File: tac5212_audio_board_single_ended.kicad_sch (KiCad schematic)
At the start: 94 parts, among them J1002 TAC5212, U1 Single Buffer - 74LVC1G125GV,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, U2 3.3v LDO - TLV74133PDBVR

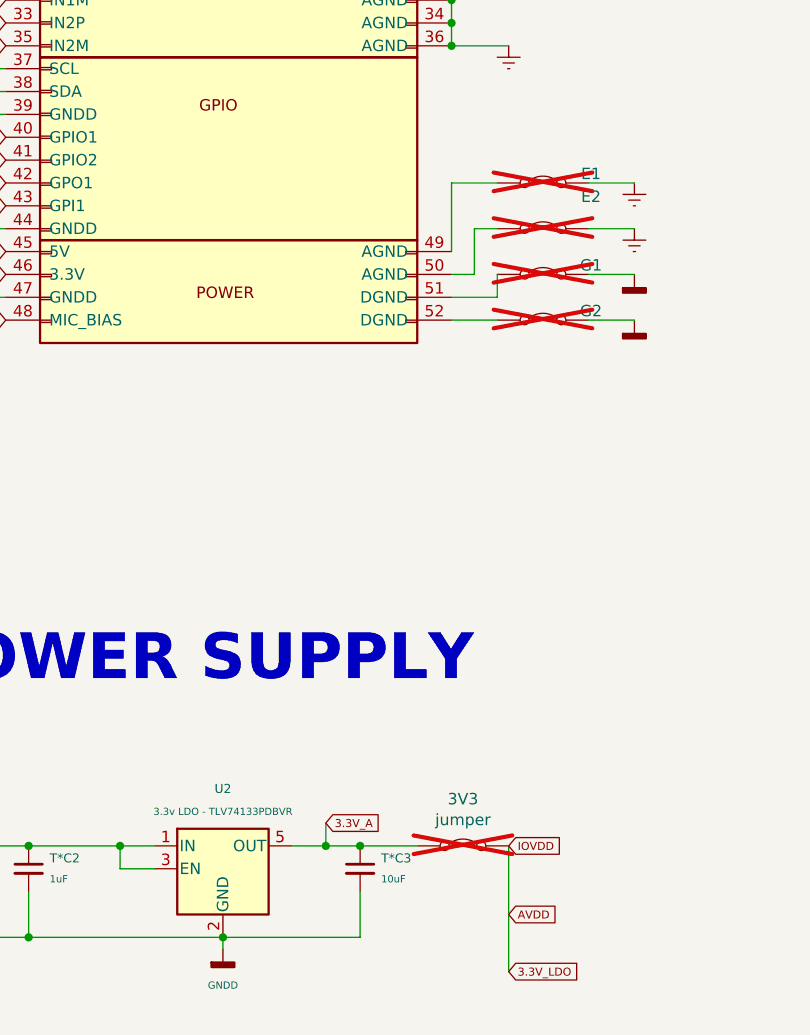
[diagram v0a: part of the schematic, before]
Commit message: UPDATE
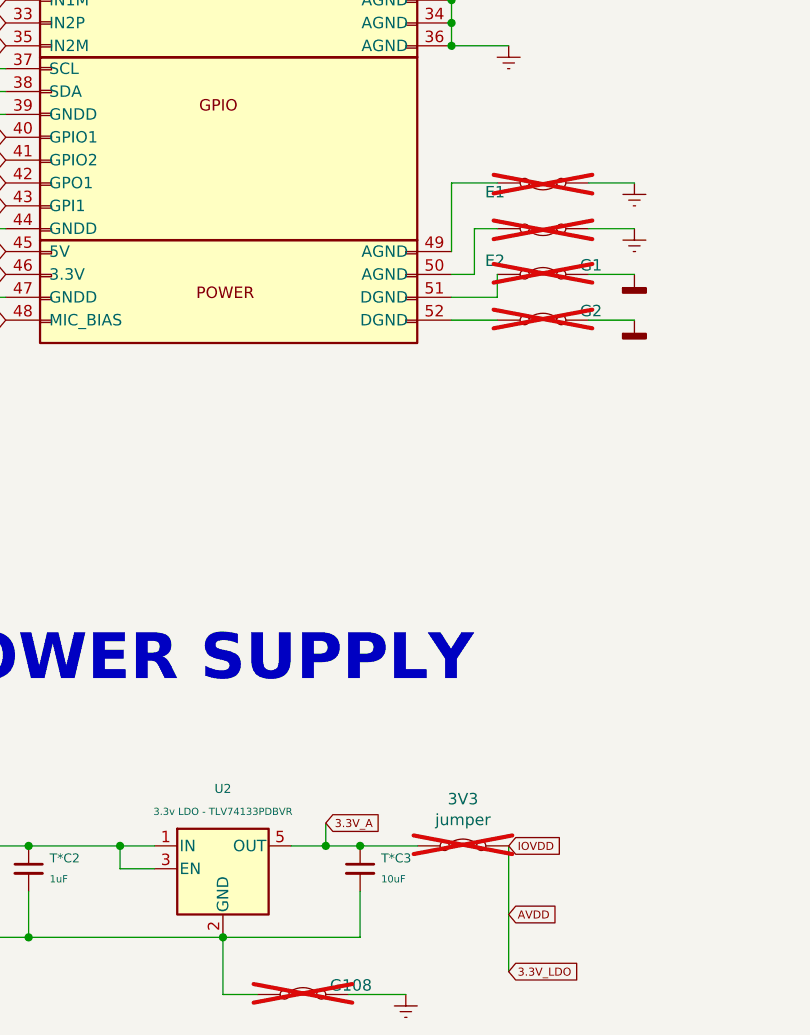
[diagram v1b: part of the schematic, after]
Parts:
- added G108: jumper, project_fp:jumper_slice, symbol proejct_lib:Jumper_2_Bridged
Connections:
- net Earth: now also E1.1 (A), E2.1 (A), G108.2 (B); no longer E1.2 (B), E2.2 (B)
- net GNDD: no longer T*C1.2, T*C2.2, T*C3.2, U2.2 (GND)
- net at board_outline1.49 (AGND): now also E1.2 (B); no longer E1.1 (A)
- net at board_outline1.50 (AGND): now also E2.2 (B); no longer E2.1 (A)
- new net: G108.1 (A), T*C1.2, T*C2.2, T*C3.2, U2.2 (GND)
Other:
- moved on the sheet: E1, E2
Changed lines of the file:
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@@
 	(wire
 		(pts
+			(xy 110.49 372.11) (xy 104.14 372.11)
+		)
+		(stroke
+			(width 0)
+			(type default)
+		)
+	)
+	(wire
+		(pts
 			(xy 218.44 168.91) (xy 222.25 168.91)
 		)
@@
 	(wire
 		(pts
-			(xy 90.17 367.03) (xy 90.17 365.76)
-		)
-		(stroke
-			(width 0)
-			(type default)
-		)
-	)
-	(wire
-		(pts
 			(xy 190.5 91.44) (xy 199.39 91.44)
 		)
@@
 	(wire
 		(pts
+			(xy 90.17 372.11) (xy 93.98 372.11)
+		)
+		(stroke
+			(width 0)
+			(type default)
+		)
+	)
+	(wire
+		(pts
 			(xy 49.53 294.64) (xy 66.04 294.64)
 		)
@@
 	(wire
 		(pts
+			(xy 90.17 372.11) (xy 90.17 365.76)
+		)
+		(stroke
+			(width 0)
+			(type default)
+		)
+	)
+	(wire
+		(pts
 			(xy 71.12 156.21) (xy 71.12 157.48)
 		)
@@
 	)
 	(symbol
+		(lib_id "proejct_lib:Earth")
+		(at 110.49 372.11 0)
+		(mirror y)
+		(unit 1)
+		(exclude_from_sim no)
+		(in_bom yes)
+		(on_board yes)
+		(dnp no)
+		(fields_autoplaced yes)
+		(property "Reference" "#PWR0108"
+			(at 110.49 378.46 0)
+			(effects
+				(font
+					(size 1 1)
+				)
+				(hide yes)
+			)
+		)
+		(property "Value" "Earth"
+			(at 110.49 375.92 0)
+			(effects
+				(font
+					(size 0.8 0.8)
+				)
+				(hide yes)
+			)
+		)
+		(property "Footprint" ""
+			(at 110.49 372.11 0)
+			(effects
+				(font
+					(size 0.8 0.8)
+				)
+				(hide yes)
+			)
+		)
+		(property "Datasheet" "~"
+			(at 110.49 372.11 0)
+			(effects
+				(font
+					(size 0.8 0.8)
+				)
+				(hide yes)
+			)
+		)
+		(property "Description" ""
+			(at 110.49 372.11 0)
+			(effects
+				(font
+					(size 1.27 1.27)
+				)
+				(hide yes)
+			)
+		)
+		(pin "1"
+		)
+		(instances
+			(project "tac5212_audio_board_single_ended"
+				(path "/8cee3af6-3893-45a9-89a4-21657973eeff"
+					(reference "#PWR0108")
+					(unit 1)
+				)
+			)
+		)
+	)
+	(symbol
 		(lib_name "Jumper_NO_Small-Device_1")
 		(lib_id "proejct_lib:Jumper_NO_Small-Device_1")
@@
 	(symbol
 		(lib_id "proejct_lib:Jumper_2_Bridged")
-		(at 125.73 287.02 0)
+		(at 125.73 287.02 180)
 		(unit 1)
 		(exclude_from_sim yes)
@@
 		(dnp yes)
 		(property "Reference" "E2"
-			(at 131.064 283.464 0)
+			(at 120.396 290.576 0)
 			(effects
 				(font
@@
 		)
 		(property "Value" "jumper"
-			(at 119.38 283.21 0)
+			(at 132.08 290.83 0)
 			(effects
 				(font
@@
 	)
 	(symbol
-		(lib_id "proejct_lib:GNDD")
-		(at 90.17 367.03 0)
-		(unit 1)
-		(exclude_from_sim no)
-		(in_bom yes)
-		(on_board yes)
-		(dnp no)
-		(fields_autoplaced yes)
-		(property "Reference" "#PWR013"
-			(at 90.17 373.38 0)
-			(effects
-				(font
-					(size 1 1)
-				)
-				(hide yes)
-			)
-		)
-		(property "Value" "GNDD"
-			(at 90.17 371.094 0)
-			(effects
-				(font
-					(size 0.8 0.8)
-				)
-			)
-		)
-		(property "Footprint" ""
-			(at 90.17 367.03 0)
-			(effects
-				(font
-					(size 0.8 0.8)
-				)
-				(hide yes)
-			)
-		)
-		(property "Datasheet" ""
-			(at 90.17 367.03 0)
-			(effects
-				(font
-					(size 0.8 0.8)
-				)
-				(hide yes)
-			)
-		)
-		(property "Description" ""
-			(at 90.17 367.03 0)
-			(effects
-				(font
-					(size 1.27 1.27)
-				)
-				(hide yes)
-			)
-		)
-		(pin "1"
-		)
-		(instances
-			(project "tac5212_audio_board_single_ended"
-				(path "/8cee3af6-3893-45a9-89a4-21657973eeff"
-					(reference "#PWR013")
-					(unit 1)
-				)
-			)
-		)
-	)
-	(symbol
 		(lib_id "proejct_lib:Jumper_NO_Small-Device")
 		(at 241.3 118.11 0)
@@
 	)
 	(symbol
+		(lib_id "proejct_lib:Jumper_2_Bridged")
+		(at 99.06 372.11 0)
+		(unit 1)
+		(exclude_from_sim yes)
+		(in_bom yes)
+		(on_board yes)
+		(dnp yes)
+		(property "Reference" "G108"
+			(at 104.394 371.094 0)
+			(effects
+				(font
+					(size 1.27 1.27)
+				)
+			)
+		)
+		(property "Value" "jumper"
+			(at 92.71 370.84 0)
+			(effects
+				(font
+					(size 1.27 1.27)
+				)
+				(hide yes)
+			)
+		)
+		(property "Footprint" "project_fp:jumper_slice"
+			(at 99.06 372.11 0)
+			(effects
+				(font
+					(size 1.27 1.27)
+				)
+				(hide yes)
+			)
+		)
+		(property "Datasheet" "~"
+			(at 99.06 372.11 0)
+			(effects
+				(font
+					(size 1.27 1.27)
+				)
+				(hide yes)
+			)
+		)
+		(property "Description" "Jumper, open"
+			(at 99.06 372.11 0)
+			(effects
+				(font
+					(size 1.27 1.27)
+				)
+				(hide yes)
+			)
+		)
+		(property "Label" "G"
+			(at 99.06 372.11 0)
+			(effects
+				(font
+					(size 1.27 1.27)
+				)
+				(hide yes)
+			)
+		)
+		(property "Package / Case" "DNP"
+			(at 99.06 372.11 0)
+			(effects
+				(font
+					(size 1.27 1.27)
+				)
+				(hide yes)
+			)
+		)
+		(property "TAC5212EVM" "n/a"
+			(at 99.06 372.11 0)
+			(effects
+				(font
+					(size 1.27 1.27)
+				)
+				(hide yes)
+			)
+		)
+		(pin "1"
+		)
+		(pin "2"
+		)
+		(instances
+			(project "tac5212_audio_board_single_ended"
+				(path "/8cee3af6-3893-45a9-89a4-21657973eeff"
+					(reference "G108")
+					(unit 1)
+				)
+			)
+		)
+	)
+	(symbol
 		(lib_id "proejct_lib:GNDD")
 		(at 144.78 162.56 0)
@@
 	(symbol
 		(lib_id "proejct_lib:Jumper_2_Bridged")
-		(at 125.73 281.94 0)
+		(at 125.73 281.94 180)
 		(unit 1)
 		(exclude_from_sim yes)
@@
 		(dnp yes)
 		(property "Reference" "E1"
-			(at 131.064 280.924 0)
+			(at 120.396 282.956 0)
 			(effects
 				(font
@@
 		)
 		(property "Value" "jumper"
-			(at 119.38 280.67 0)
+			(at 132.08 283.21 0)
 			(effects
 				(font

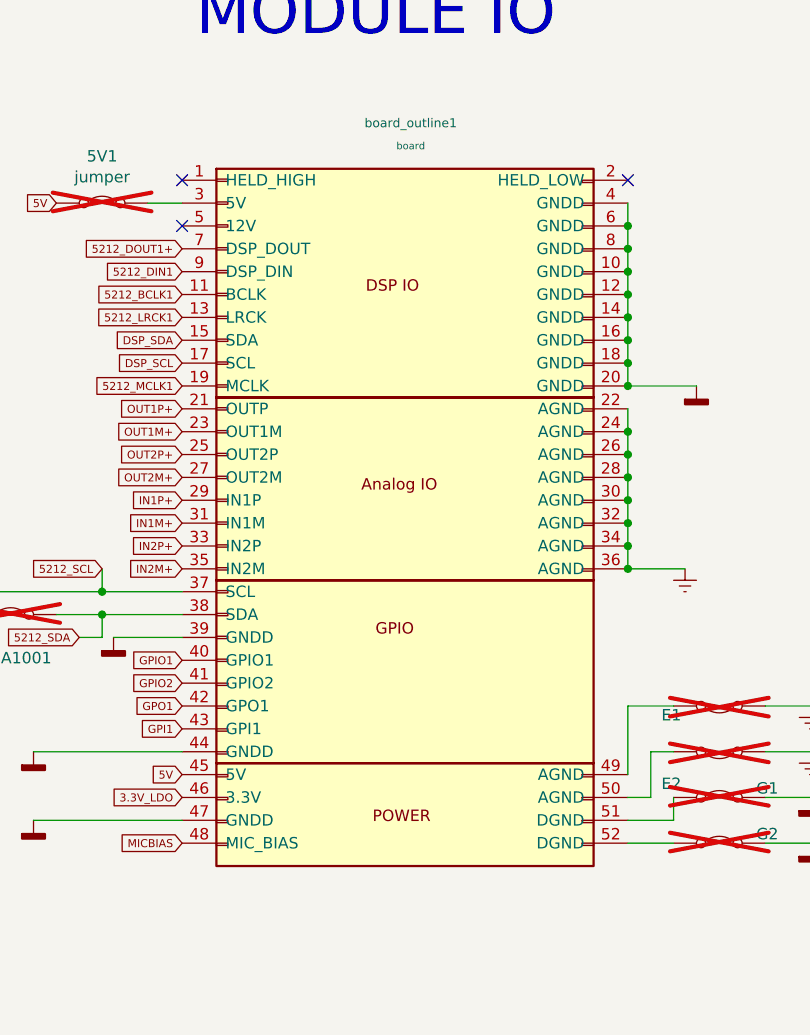
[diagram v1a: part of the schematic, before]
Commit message: update
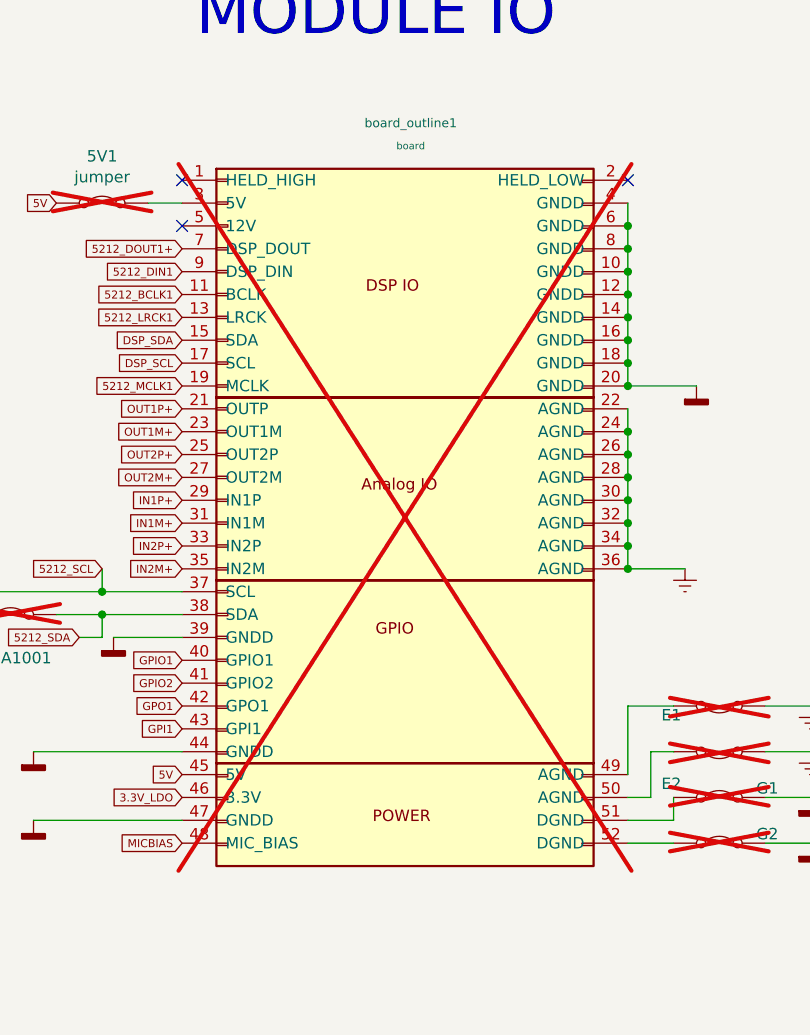
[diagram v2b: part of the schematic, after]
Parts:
- board_outline1: now not fitted
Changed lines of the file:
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@@
 		(in_bom yes)
 		(on_board yes)
-		(dnp no)
+		(dnp yes)
 		(property "Reference" "board_outline1"
 			(at 91.44 217.17 0)
